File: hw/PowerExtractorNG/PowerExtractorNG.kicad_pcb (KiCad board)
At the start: 2 copper layers, 69.2 x 45.7 mm, 11 parts, among them J1 INPUT RECTIFIED, J2 OUTPUT, Q1 IRFB4110

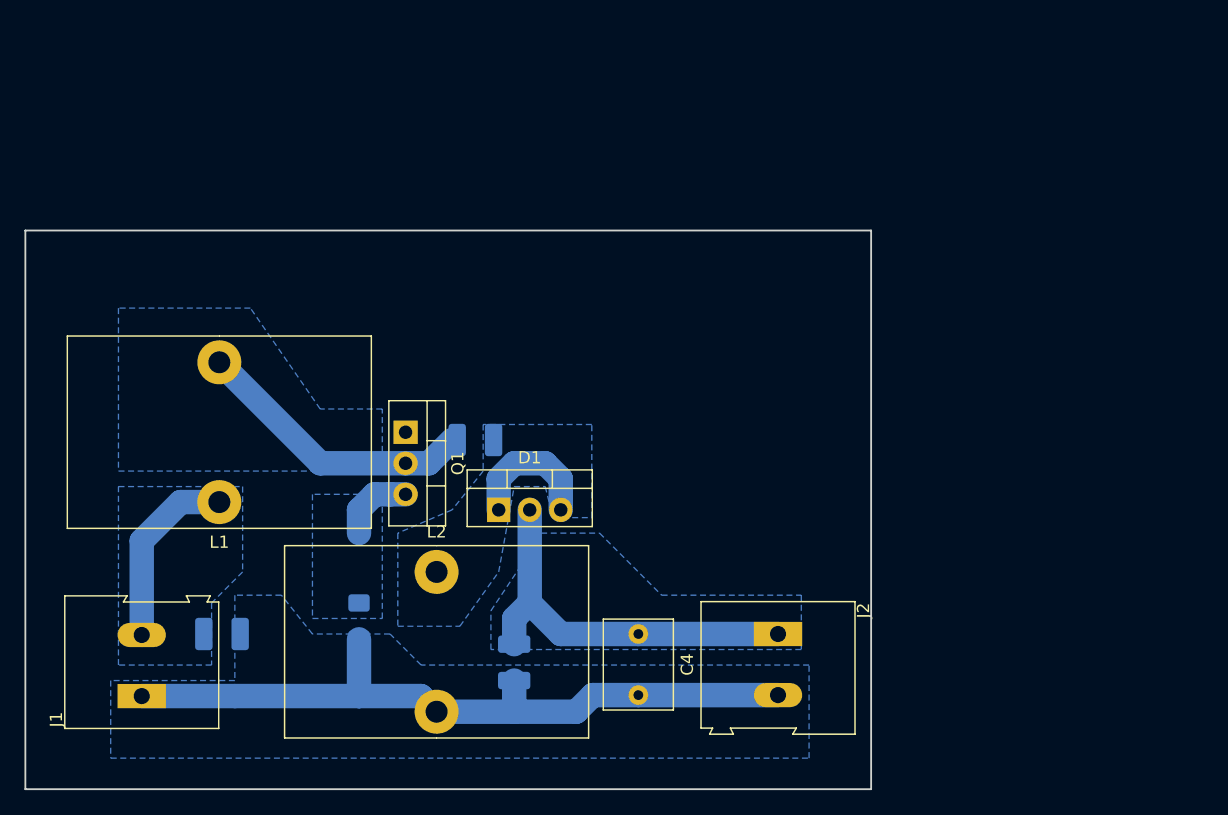
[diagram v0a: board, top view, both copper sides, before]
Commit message: Done
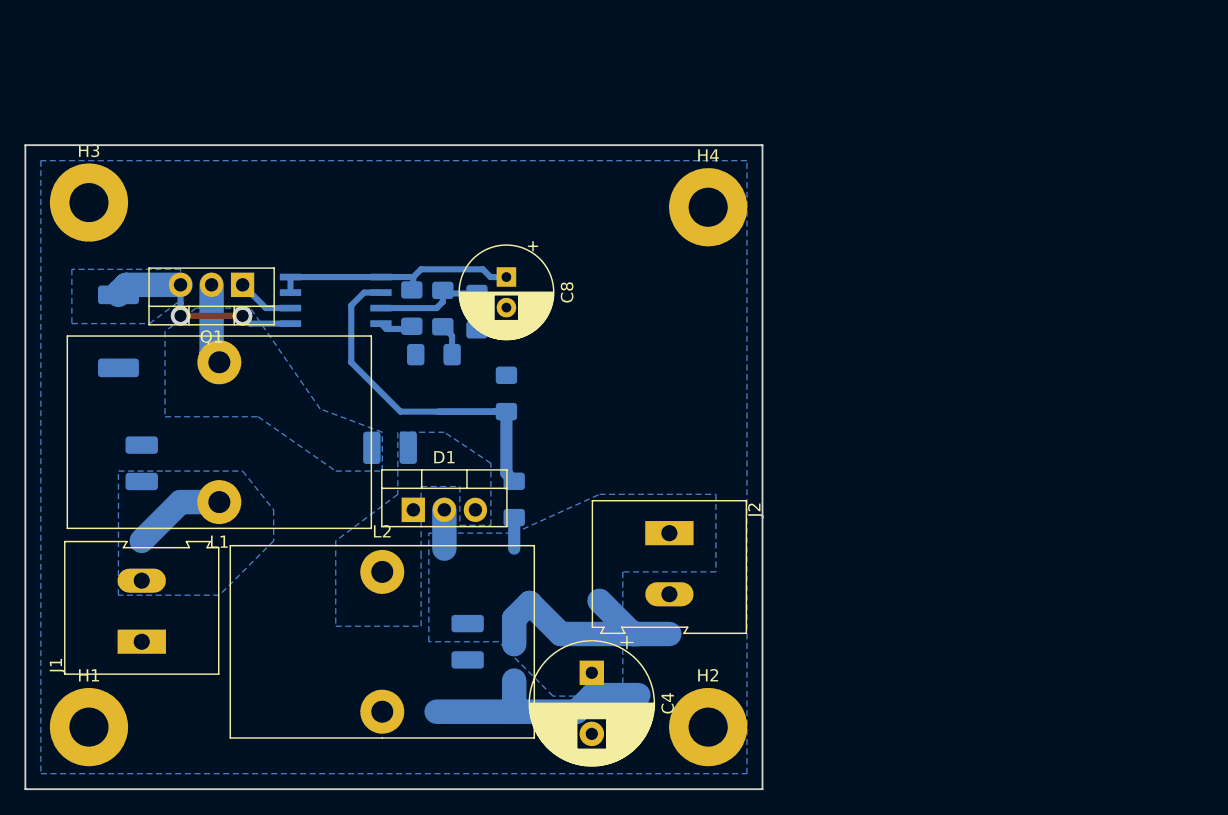
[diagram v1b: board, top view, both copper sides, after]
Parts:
- added C5: 220pF, Capacitor_SMD:C_1206_3216Metric_Pad1.42x1.75mm_HandSolder, B.Cu at (136.7, 77.8)
- added C6: 15nF, Capacitor_SMD:C_1206_3216Metric_Pad1.42x1.75mm_HandSolder, B.Cu at (133.1, 81.3)
- added C7: 100nF, Capacitor_SMD:C_1206_3216Metric_Pad1.42x1.75mm_HandSolder, B.Cu at (131.3, 77.5)
- added C8: 22uF, Capacitor_THT:CP_Radial_D7.5mm_P2.50mm, F.Cu at (139.1, 74.9)
- added H1: MountingHole_Pad, MountingHole:MountingHole_3.2mm_M3_Pad, F.Cu at (104.9, 111.8)
- added H2: MountingHole_Pad, MountingHole:MountingHole_3.2mm_M3_Pad, F.Cu at (155.6, 111.8)
- added H3: MountingHole_Pad, MountingHole:MountingHole_3.2mm_M3_Pad, F.Cu at (104.9, 68.8)
- added H4: MountingHole_Pad, MountingHole:MountingHole_3.2mm_M3_Pad, F.Cu at (155.6, 69.2)
- added R2: 75k, Resistor_SMD:R_1206_3216Metric_Pad1.42x1.75mm_HandSolder, B.Cu at (133.9, 77.5)
- added R3: 120k**, Resistor_SMD:R_1206_3216Metric_Pad1.42x1.75mm_HandSolder, B.Cu at (139.7, 93.1)
- added R4: 10k, Resistor_SMD:R_1206_3216Metric_Pad1.42x1.75mm_HandSolder, B.Cu at (139.1, 84.5)
- added U1: LT1619, Package_SO:SO-8_5.3x6.2mm_P1.27mm, B.Cu at (125.1, 76.8)
- C4: footprint Capacitor_THT:C_Rect_L7.2mm_W5.5mm_P5.00mm_FKS2_FKP2_MKS2_MKP2 -> Capacitor_THT:CP_Radial_D10.0mm_P5.00mm
- R1: value 0R1 -> 0R01; footprint Resistor_SMD:R_1206_3216Metric_Pad1.42x1.75mm_HandSolder -> Resistor_SMD:R_2512_6332Metric_Pad1.52x3.35mm_HandSolder
- moved R1 30.8 mm to (107.3, 79.4)
- moved Q1 18.0 mm to (117.5, 75.6), turned to 180 degrees
- moved C1 15.4 mm to (109.2, 90.2), turned to 90 degrees
- moved J2 12.1 mm to (152.4, 95.9)
- moved C2 7.01 mm to (129.5, 88.9)
- moved D1 6.99 mm to (131.4, 94.0)
- moved C4 4.96 mm to (146.1, 107.3)
- moved J1 4.44 mm to (109.2, 104.8)
- moved L2 4.44 mm to (128.9, 99.1)
- moved C3 4.17 mm to (135.9, 104.8)
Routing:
- net Net-(C1-Pad2): track 60.4 -> 22.5 mm
- net Net-(R3-Pad2): track 0.00 -> 33.4 mm
- net Net-(C7-Pad1): track 0.00 -> 21.5 mm
- net Net-(C2-Pad2): track 23.3 -> 6.60 mm
- net Net-(C2-Pad1): track 11.2 -> 0.00 mm
- net Net-(Q1-Pad3): track 6.24 -> 17.4 mm, vias 0 -> 2
- net Net-(C5-Pad1): track 0.00 -> 9.12 mm
- net Net-(C1-Pad1): track 15.4 -> 7.67 mm
- net Net-(C3-Pad1): track 32.9 -> 26.4 mm
- net Net-(Q1-Pad1): track 0.00 -> 4.71 mm
- net Net-(C6-Pad1): track 0.00 -> 2.60 mm
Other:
- board size 69.2 x 45.7 mm -> 60.3 x 52.7 mm

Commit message: PE2020
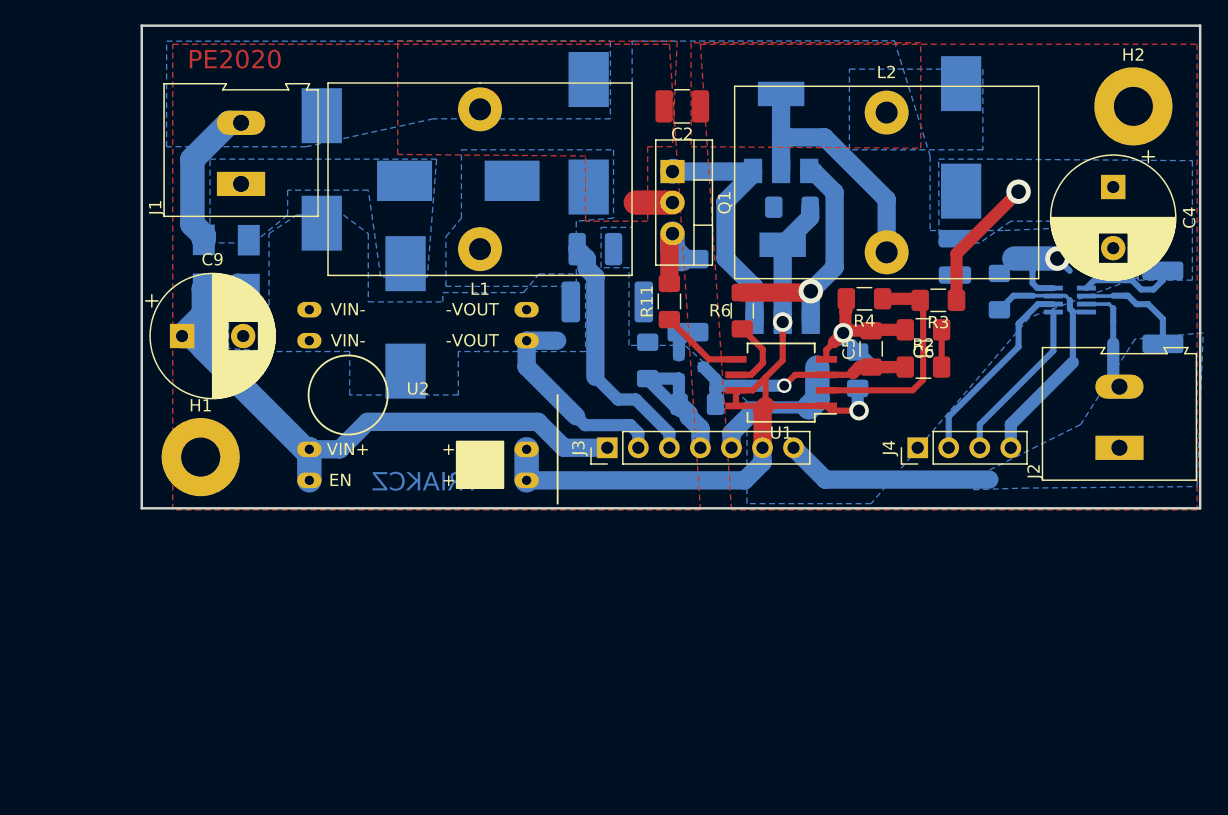
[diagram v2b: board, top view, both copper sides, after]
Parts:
- removed H3, H4: MountingHole_Pad, MountingHole:MountingHole_3.2mm_M3_Pad
- added C10: 100nF, Capacitor_SMD:C_1206_3216Metric_Pad1.42x1.75mm_HandSolder, B.Cu at (179.4, 76.1)
- added C9: 100u/63V, Capacitor_THT:CP_Radial_D10.0mm_P5.00mm, F.Cu at (112.5, 79.8)
- added D2: 1N4007, Diode_SMD:D_SMA, B.Cu at (114.3, 73.9)
- added D3: SS510, Diode_SMD:D_SMC_Handsoldering, B.Cu at (145.8, 63.2)
- added D4: SS510, Diode_SMD:D_SMC_Handsoldering, B.Cu at (124.0, 66.1)
- added D5: SS510, Diode_SMD:D_SMC_Handsoldering, B.Cu at (135.1, 67.1)
- added D6: SS510, Diode_SMD:D_SMC_Handsoldering, B.Cu at (130.8, 78.2)
- added D7: SS510, Diode_SMD:D_SMC_Handsoldering, B.Cu at (176.3, 63.5)
- added J3: Control, Connector_PinHeader_2.54mm:PinHeader_1x07_P2.54mm_Vertical, F.Cu at (147.3, 88.9)
- added J4: I2C, Connector_PinHeader_2.54mm:PinHeader_1x04_P2.54mm_Vertical, F.Cu at (172.7, 88.9)
- added NT1: Net-Tie_2, NetTie:NetTie-2_SMD_Pad0.5mm, B.Cu at (189.2, 75.2)
- added NT2: Net-Tie_2, NetTie:NetTie-2_SMD_Pad0.5mm, B.Cu at (189.2, 76.5)
- added NT3: Net-Tie_2, NetTie:NetTie-2_SMD_Pad0.5mm, B.Cu at (188.7, 78.0)
- added NT4: Net-Tie_2, NetTie:NetTie-2_SMD_Pad0.5mm, B.Cu at (185.4, 80.6)
- added NT5: Net-Tie_2, NetTie:NetTie-2_SMD_Pad0.5mm, B.Cu at (182.1, 74.9)
- added Q2: BCP56, Package_TO_SOT_SMD:SOT-223-3_TabPin2, B.Cu at (161.7, 75.4)
- added Q3: BCP53, Package_TO_SOT_SMD:SOT-223-3_TabPin2, B.Cu at (161.5, 63.1)
- added Q4: BC847, Package_TO_SOT_SMD:SOT-23, B.Cu at (154.2, 82.3)
- added R11: TBD (BURST mode), Resistor_SMD:R_1206_3216Metric_Pad1.42x1.75mm_HandSolder, F.Cu at (152.4, 76.9)
- added R5: 0R05, Resistor_SMD:R_2512_6332Metric_Pad1.52x3.35mm_HandSolder, B.Cu at (147.3, 77.0)
- added R6: 100R, Resistor_SMD:R_1206_3216Metric_Pad1.42x1.75mm_HandSolder, F.Cu at (158.4, 77.7)
- added R7: 330k, Resistor_SMD:R_1206_3216Metric_Pad1.42x1.75mm_HandSolder, B.Cu at (154.7, 85.3)
- added R8: 100k, Resistor_SMD:R_1206_3216Metric_Pad1.42x1.75mm_HandSolder, B.Cu at (150.6, 81.8)
- added R9: 0R05, Resistor_SMD:R_2512_6332Metric_Pad1.52x3.35mm_HandSolder, B.Cu at (192.8, 77.4)
- added U2: DM01module, triakcz_modules:DM01_mod_THT, F.Cu at (131.8, 84.6)
- added U3: INA219_SOT23-8, Package_TO_SOT_SMD:SOT-23-8_Handsoldering, B.Cu at (185.2, 76.8)
- C2, C5, C6, R2, R3, R4, U1: moved to F.Cu
- C8: value 22uF -> 100nF; footprint Capacitor_THT:CP_Radial_D7.5mm_P2.50mm -> Capacitor_SMD:C_1206_3216Metric_Pad1.42x1.75mm_HandSolder; moved to B.Cu
- D1: value D_x2_KCom_AKA -> 1N4007; footprint Package_TO_SOT_THT:TO-220-3_Vertical -> Diode_SMD:D_SMA; moved to B.Cu
- J1: value INPUT RECTIFIED -> INPUT AC
- R1: value 0R01 -> 0R05
- moved H2 61.6 mm to (190.4, 61.0)
- moved C4 58.3 mm to (188.7, 67.6)
- moved L2 55.8 mm to (170.2, 61.5)
- moved C3 50.8 mm to (175.8, 73.3)
- moved R1 46.7 mm to (153.9, 76.5)
- moved C1 41.0 mm to (146.3, 72.6), turned to 0 degrees
- moved C6 40.1 mm to (173.2, 79.2)
- moved R2 39.6 mm to (173.2, 82.3), turned to 0 degrees
- moved R3 38.3 mm to (174.4, 76.8), turned to 180 degrees
- moved J1 38.3 mm to (117.3, 67.3)
- moved J2 37.5 mm to (189.2, 88.9), turned to 90 degrees
- moved U1 37.1 mm to (161.5, 83.6)
- moved C2 36.8 mm to (153.5, 61.0)
- moved Q1 36.4 mm to (152.7, 66.3), turned to 270 degrees
- moved C5 32.4 mm to (168.9, 80.8), turned to 90 degrees
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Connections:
- net Net-(C7-Pad1) renamed /9VDC
- C1 pad 1: Net-(C1-Pad1) -> /MAIN_RECT
- C1 pad 2: Net-(C1-Pad2) -> /GND_SENSE
- C3 pad 2: Net-(C1-Pad2) -> /GND_SENSE
- C4 pad 2: Net-(C1-Pad2) -> /GND_SENSE
- C5 pad 2: Net-(C1-Pad2) -> /GND_SENSE
- C6 pad 2: Net-(C1-Pad2) -> /GND_SENSE
- C7 pad 2: Net-(C1-Pad2) -> /GND_SENSE
- C8 pad 2: Net-(C1-Pad2) -> /GND_SENSE
- D1 pad 1: Net-(C2-Pad1) -> /AUX_RECT
- D1 pad 2: Net-(C3-Pad1) -> Net-(D1-Pad2)
- H1 pad 1: Net-(C1-Pad2) -> (no net)
- H2 pad 1: Net-(C1-Pad2) -> (no net)
- J1 pad 1: Net-(C1-Pad2) -> Net-(D1-Pad2)
- J1 pad 2: Net-(C1-Pad1) -> Net-(D2-Pad2)
- J2 pad 1: Net-(C3-Pad1) -> /OUT+
- J2 pad 2: Net-(C1-Pad2) -> /GND_SENSE
- L1 pad 1: Net-(C1-Pad1) -> /MAIN_RECT
- L2 pad 2: Net-(C1-Pad2) -> /GND_SENSE
- R1 pad 2: Net-(C1-Pad2) -> /GND_SENSE
- R4 pad 2: Net-(C1-Pad2) -> /GND_SENSE
- U1 pad 4: Net-(C1-Pad2) -> /GND_SENSE
- U1 pad 5: Net-(Q1-Pad3) -> Net-(R11-Pad1)
- U1 pad 6: Net-(Q1-Pad1) -> Net-(R6-Pad1)
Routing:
- net /GND_SENSE: track 0.00 -> 66.1 mm, vias 0 -> 2
- net /AUX_RECT: track 0.00 -> 55.8 mm
- net /9VDC: track 21.5 -> 62.7 mm, vias 0 -> 2
- net /OUT+: track 0.00 -> 23.0 mm
- net Net-(C1-Pad2): track 22.5 -> 0.00 mm
- net /MAIN_RECT: track 0.00 -> 20.2 mm
- net Net-(Q2-Pad1): track 0.00 -> 20.1 mm, vias 0 -> 1
- net /GND_RECT: track 0.00 -> 17.2 mm
- net Net-(Q1-Pad1): track 4.71 -> 21.2 mm
- net /SDA: track 0.00 -> 16.0 mm
- net Net-(R3-Pad2): track 33.4 -> 17.7 mm
- net /SCL: track 0.00 -> 13.6 mm
- net /VCOMP_CTRL: track 0.00 -> 13.1 mm
- net Net-(D2-Pad2): track 0.00 -> 12.2 mm
- net Net-(C3-Pad1): track 26.4 -> 15.4 mm, vias 0 -> 1
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- added copper zone on B.Cu, net /GND_RECT
- added copper zone on F.Cu, net /GND_RECT
- added copper zone on B.Cu, net /GND_SENSE
- added copper zone on F.Cu, net /GND_SENSE
- added copper zone on B.Cu, net /MAIN_RECT
- added copper zone on B.Cu, net /OUT+
- added copper zone on F.Cu, net Net-(C2-Pad1)
- added copper zone on F.Cu, net Net-(C2-Pad2)
- added copper zone on B.Cu, net Net-(D1-Pad2)
- added copper zone on B.Cu, net Net-(D2-Pad2)
- removed copper zone on B.Cu, net Net-(C1-Pad1)
- removed copper zone on B.Cu, net Net-(C1-Pad2)
- removed copper zone on B.Cu, net Net-(C2-Pad2)
- removed copper zone on B.Cu, net Net-(Q1-Pad3)
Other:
- board size 60.3 x 52.7 mm -> 86.6 x 39.5 mm
- net class Signal added: clearance 0.1, trace_width 0.3, via_dia 1, via_drill 0.8
- rule solder_mask_min_width: 0.25 -> 0.05
- rule trace_min: 0.5 -> 0.3
- board text added: "PE2020"
- board text added: "TRIAKCZ"
